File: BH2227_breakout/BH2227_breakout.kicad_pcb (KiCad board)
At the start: 2 copper layers, 22.9 x 25.4 mm, 5 parts, among them J1 Conn_01x04_Male, J2 Conn_01x05_Male, U1 BH2227FV

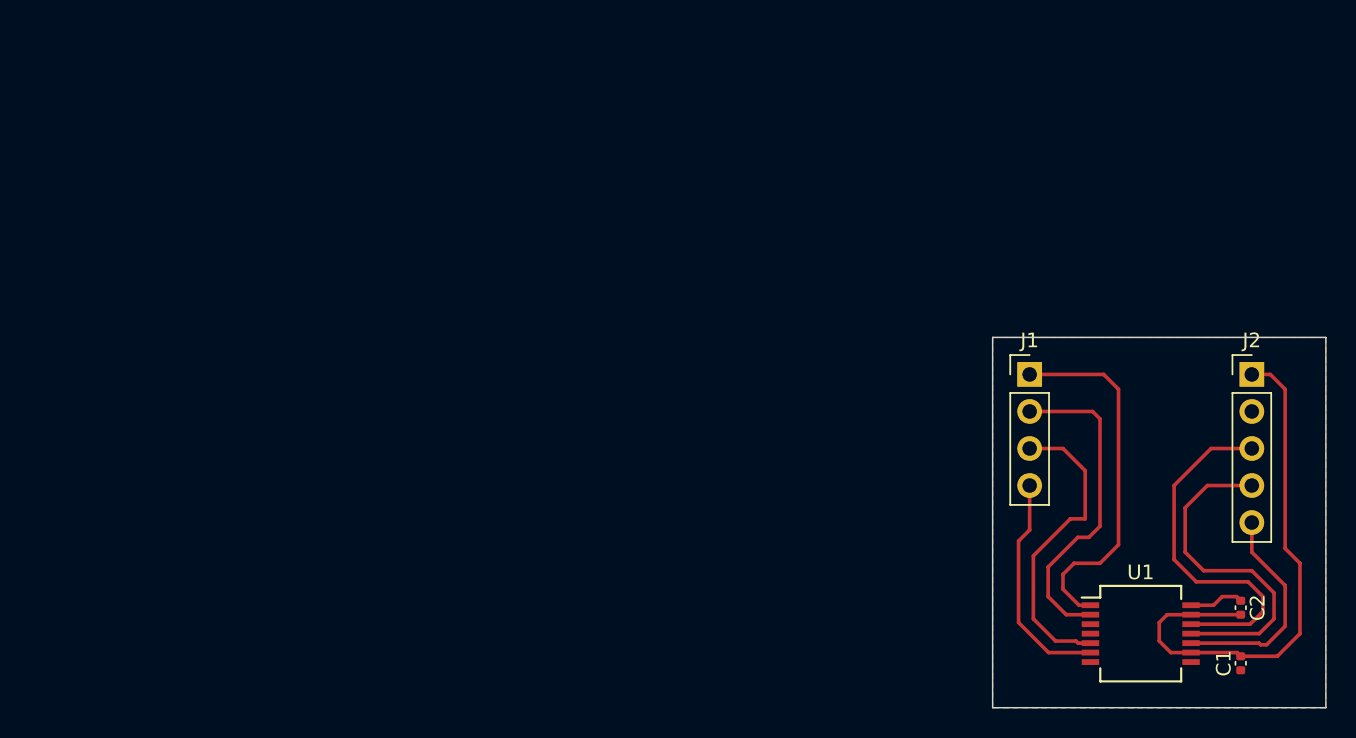
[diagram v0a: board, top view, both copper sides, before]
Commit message: update schematic for eurorack_to_3v, add BH2227 pcb layout
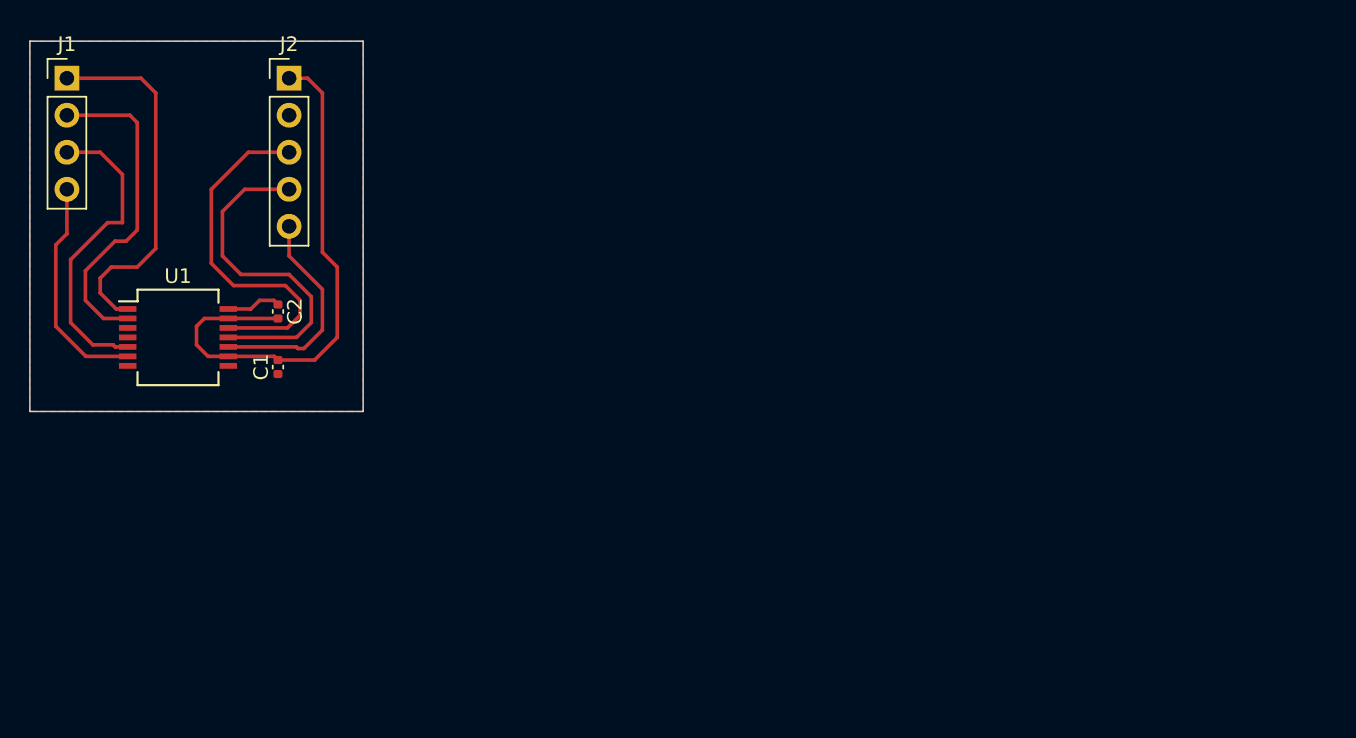
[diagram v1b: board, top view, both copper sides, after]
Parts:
- moved C1 69.1 mm to (75.4, 65.5)
- moved C2 69.1 mm to (75.4, 61.7)
- moved J2 69.1 mm to (76.2, 45.7)
- moved J1 69.1 mm to (61.0, 45.7)
- moved U1 69.1 mm to (68.6, 63.5)
